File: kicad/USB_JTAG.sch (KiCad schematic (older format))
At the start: 23 parts, among them J1 USB_B, U4 NFM18PS, U5 WE-TVS-824011, U6 FT2232D, U7 6MHz_Crystal, U8 AT93C46DN-SH

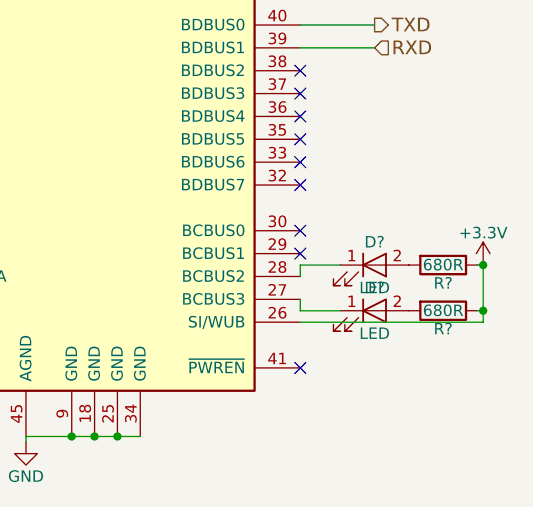
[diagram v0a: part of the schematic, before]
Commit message: Layout changes [In progress]
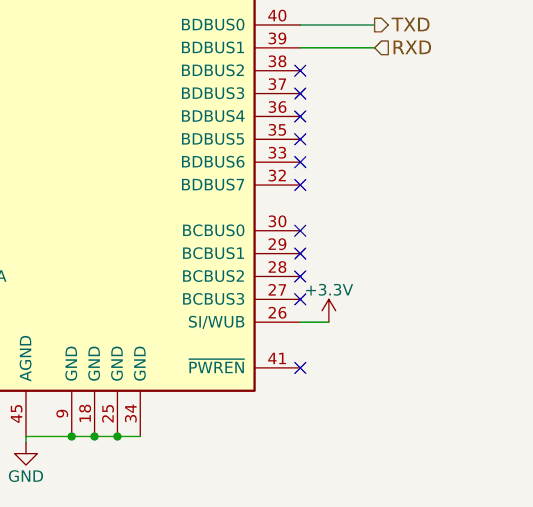
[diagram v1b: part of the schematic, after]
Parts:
- removed D? (x2): LED, Footprints_LJ:Mini_TopLed_SMD, symbol LED
- removed R? (x2): 680R, Resistors_SMD:R_0603_HandSoldering, symbol R
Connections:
- no-connect marks 19 -> 21
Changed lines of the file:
@@
 $EndComp
 $Comp
-L GND #PWR084
+L GND #PWR082
 U 1 1 595D2BC3
 P 1400 3350
-F 0 "#PWR084" H 1400 3100 50  0001 C CNN
+F 0 "#PWR082" H 1400 3100 50  0001 C CNN
 F 1 "GND" H 1400 3200 50  0000 C CNN
 F 2 "" H 1400 3350 50  0001 C CNN
@@
 $EndComp
 $Comp
-L GND #PWR085
+L GND #PWR083
 U 1 1 595D2BF4
 P 5975 5550
-F 0 "#PWR085" H 5975 5300 50  0001 C CNN
+F 0 "#PWR083" H 5975 5300 50  0001 C CNN
 F 1 "GND" H 5975 5400 50  0000 C CNN
 F 2 "" H 5975 5550 50  0001 C CNN
@@
 $EndComp
 $Comp
-L GND #PWR086
+L GND #PWR084
 U 1 1 595D2BFA
 P 5375 5025
-F 0 "#PWR086" H 5375 4775 50  0001 C CNN
+F 0 "#PWR084" H 5375 4775 50  0001 C CNN
 F 1 "GND" H 5375 4875 50  0000 C CNN
 F 2 "" H 5375 5025 50  0001 C CNN
@@
 $EndComp
 $Comp
-L GND #PWR087
+L GND #PWR085
 U 1 1 595D2C07
 P 5075 2425
-F 0 "#PWR087" H 5075 2175 50  0001 C CNN
+F 0 "#PWR085" H 5075 2175 50  0001 C CNN
 F 1 "GND" H 5075 2275 50  0000 C CNN
 F 2 "" H 5075 2425 50  0001 C CNN
@@
 $EndComp
 $Comp
-L GND #PWR088
+L GND #PWR086
 U 1 1 595D2C1A
 P 5450 2025
-F 0 "#PWR088" H 5450 1775 50  0001 C CNN
+F 0 "#PWR086" H 5450 1775 50  0001 C CNN
 F 1 "GND" H 5450 1875 50  0000 C CNN
 F 2 "" H 5450 2025 50  0001 C CNN
@@
 $EndComp
 $Comp
-L +3.3V #PWR089
+L +3.3V #PWR087
 U 1 1 595E0732
 P 6375 1825
-F 0 "#PWR089" H 6375 1675 50  0001 C CNN
+F 0 "#PWR087" H 6375 1675 50  0001 C CNN
 F 1 "+3.3V" H 6375 1965 50  0000 C CNN
 F 2 "" H 6375 1825 50  0001 C CNN
@@
 $EndComp
 $Comp
-L GND #PWR090
+L GND #PWR088
 U 1 1 595E26E9
 P 2800 2450
-F 0 "#PWR090" H 2800 2200 50  0001 C CNN
+F 0 "#PWR088" H 2800 2200 50  0001 C CNN
 F 1 "GND" H 2800 2300 50  0000 C CNN
 F 2 "" H 2800 2450 50  0001 C CNN
@@
 $EndComp
 $Comp
-L GND #PWR091
+L GND #PWR089
 U 1 1 595E2C1D
 P 2075 3400
-F 0 "#PWR091" H 2075 3150 50  0001 C CNN
+F 0 "#PWR089" H 2075 3150 50  0001 C CNN
 F 1 "GND" H 2075 3250 50  0000 C CNN
 F 2 "" H 2075 3400 50  0001 C CNN
@@
 $EndComp
 $Comp
-L GND #PWR092
+L GND #PWR090
 U 1 1 595E6BEC
 P 2200 2250
-F 0 "#PWR092" H 2200 2000 50  0001 C CNN
+F 0 "#PWR090" H 2200 2000 50  0001 C CNN
 F 1 "GND" H 2200 2100 50  0000 C CNN
 F 2 "" H 2200 2250 50  0001 C CNN
@@
 $EndComp
 $Comp
-L GND #PWR093
+L GND #PWR091
 U 1 1 5961A2DE
 P 2400 3400
-F 0 "#PWR093" H 2400 3150 50  0001 C CNN
+F 0 "#PWR091" H 2400 3150 50  0001 C CNN
 F 1 "GND" H 2400 3250 50  0000 C CNN
 F 2 "" H 2400 3400 50  0001 C CNN
@@
 ~RESET
 $Comp
-L +3.3V #PWR094
+L +3.3V #PWR092
 U 1 1 5964E324
 P 3850 4225
-F 0 "#PWR094" H 3850 4075 50  0001 C CNN
+F 0 "#PWR092" H 3850 4075 50  0001 C CNN
 F 1 "+3.3V" H 3850 4365 50  0000 C CNN
 F 2 "" H 3850 4225 50  0001 C CNN
@@
 $EndComp
 $Comp
-L +3.3V #PWR095
+L +3.3V #PWR093
 U 1 1 5964E7A5
 P 2750 4650
-F 0 "#PWR095" H 2750 4500 50  0001 C CNN
+F 0 "#PWR093" H 2750 4500 50  0001 C CNN
 F 1 "+3.3V" H 2750 4790 50  0000 C CNN
 F 2 "" H 2750 4650 50  0001 C CNN
@@
 $EndComp
 $Comp
-L GND #PWR096
+L GND #PWR094
 U 1 1 5964E8AB
 P 2750 4950
-F 0 "#PWR096" H 2750 4700 50  0001 C CNN
+F 0 "#PWR094" H 2750 4700 50  0001 C CNN
 F 1 "GND" H 2750 4800 50  0000 C CNN
 F 2 "" H 2750 4950 50  0001 C CNN
@@
 $EndComp
 $Comp
-L +5V #PWR097
+L +5V #PWR095
 U 1 1 5968BBC0
 P 2075 1925
-F 0 "#PWR097" H 2075 1775 50  0001 C CNN
+F 0 "#PWR095" H 2075 1775 50  0001 C CNN
 F 1 "+5V" H 2075 2065 50  0000 C CNN
 F 2 "" H 2075 1925 50  0001 C CNN
@@
 $EndComp
 $Comp
-L +5V #PWR098
+L +5V #PWR096
 U 1 1 596B00B1
 P 6125 1700
-F 0 "#PWR098" H 6125 1550 50  0001 C CNN
+F 0 "#PWR096" H 6125 1550 50  0001 C CNN
 F 1 "+5V" H 6125 1840 50  0000 C CNN
 F 2 "" H 6125 1700 50  0001 C CNN
@@
 $EndComp
 $Comp
-L +5V #PWR099
+L +5V #PWR097
 U 1 1 596CAD7A
 P 4950 1675
-F 0 "#PWR099" H 4950 1525 50  0001 C CNN
+F 0 "#PWR097" H 4950 1525 50  0001 C CNN
 F 1 "+5V" H 4950 1815 50  0000 C CNN
 F 2 "" H 4950 1675 50  0001 C CNN
@@
 Connection ~ 4550 4325
 $Comp
-L GND #PWR0100
+L GND #PWR098
 U 1 1 5973DDBE
 P 4550 4350
-F 0 "#PWR0100" H 4550 4100 50  0001 C CNN
+F 0 "#PWR098" H 4550 4100 50  0001 C CNN
 F 1 "GND" H 4550 4200 50  0000 C CNN
 F 2 "" H 4550 4350 50  0001 C CNN
@@
 	7175 3525 7350 3525
 $Comp
-L +3.3V #PWR?
+L +3.3V #PWR099
 U 1 1 59BBED1D
 P 7350 3525
-F 0 "#PWR?" H 7350 3375 50  0001 C CNN
+F 0 "#PWR099" H 7350 3375 50  0001 C CNN
 F 1 "+3.3V" H 7350 3665 50  0000 C CNN
 F 2 "" H 7350 3525 50  0001 C CNN
@@
 	1    0    0    -1
 $EndComp
-Wire Wire Line
-	7975 4775 7950 4775
-$Comp
-L R R?
-U 1 1 59BBFFB0
-P 7800 4775
-F 0 "R?" V 7880 4775 50  0000 C CNN
-F 1 "680R" V 7800 4775 50  0000 C CNN
-F 2 "Resistors_SMD:R_0603_HandSoldering" V 7730 4775 50  0001 C CNN
-F 3 "" H 7800 4775 50  0001 C CNN
-	1    7800 4775
-	0    1    1    0
-$EndComp
-$Comp
-L LED D?
-U 1 1 59BBFFB9
-P 7500 4975
-F 0 "D?" H 7500 5075 50  0000 C CNN
-F 1 "LED" H 7500 4875 50  0000 C CNN
-F 2 "Footprints_LJ:Mini_TopLed_SMD" H 7500 4975 50  0001 C CNN
-F 3 "" H 7500 4975 50  0001 C CNN
-	1    7500 4975
-	1    0    0    -1
-$EndComp
-Wire Wire Line
-	7975 4975 7950 4975
-$Comp
-L R R?
-U 1 1 59BBFFC7
-P 7800 4975
-F 0 "R?" V 7880 4975 50  0000 C CNN
-F 1 "680R" V 7800 4975 50  0000 C CNN
-F 2 "Resistors_SMD:R_0603_HandSoldering" V 7730 4975 50  0001 C CNN
-F 3 "" H 7800 4975 50  0001 C CNN
-	1    7800 4975
-	0    1    1    0
-$EndComp
-$Comp
-L LED D?
-U 1 1 59BBFFA2
-P 7500 4775
-F 0 "D?" H 7500 4875 50  0000 C CNN
-F 1 "LED" H 7500 4675 50  0000 C CNN
-F 2 "Footprints_LJ:Mini_TopLed_SMD" H 7500 4775 50  0001 C CNN
-F 3 "" H 7500 4775 50  0001 C CNN
-	1    7500 4775
-	1    0    0    -1
-$EndComp
-Wire Wire Line
-	7175 4775 7175 4825
-Wire Wire Line
-	7175 4925 7175 4975
-$Comp
-L +3.3V #PWR?
-U 1 1 59BC15FC
-P 7975 4775
-F 0 "#PWR?" H 7975 4625 50  0001 C CNN
-F 1 "+3.3V" H 7975 4915 50  0000 C CNN
-F 2 "" H 7975 4775 50  0001 C CNN
-F 3 "" H 7975 4775 50  0001 C CNN
-	1    7975 4775
-	1    0    0    -1
-$EndComp
-Wire Wire Line
-	7175 4975 7350 4975
-Wire Wire Line
-	7175 4775 7350 4775
-Wire Wire Line
-	7975 4775 7975 5025
-Connection ~ 7975 4775
-Wire Wire Line
-	7975 5025 7175 5025
-Connection ~ 7975 4975
+NoConn ~ 7175 4825
+NoConn ~ 7175 4925
+Wire Wire Line
+	7175 5025 7300 5025
+$Comp
+L +3.3V #PWR0100
+U 1 1 59C1476A
+P 7300 5025
+F 0 "#PWR0100" H 7300 4875 50  0001 C CNN
+F 1 "+3.3V" H 7300 5165 50  0000 C CNN
+F 2 "" H 7300 5025 50  0001 C CNN
+F 3 "" H 7300 5025 50  0001 C CNN
+	1    7300 5025
+	1    0    0    -1
+$EndComp
 $EndSCHEMATC

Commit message: Remove design errors and changes some footprints [to review]
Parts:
- U7: footprint Crystals:Crystal_HC49-U_Vertical -> Crystals:Crystal_SMD_HC49-SD
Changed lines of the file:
@@
 $EndComp
 $Comp
-L GND #PWR026
+L GND #PWR027
 U 1 1 595D2BC3
 P 1400 3350
-F 0 "#PWR026" H 1400 3100 50  0001 C CNN
+F 0 "#PWR027" H 1400 3100 50  0001 C CNN
 F 1 "GND" H 1400 3200 50  0000 C CNN
 F 2 "" H 1400 3350 50  0001 C CNN
@@
 F 0 "U7" V 5625 4550 60  0000 C CNN
 F 1 "6MHz_Crystal" V 5550 4350 60  0000 C CNN
-F 2 "Crystals:Crystal_HC49-U_Vertical" H 5400 4200 60  0001 C CNN
+F 2 "Crystals:Crystal_SMD_HC49-SD" H 5400 4200 60  0001 C CNN
 F 3 "" H 5400 4200 60  0001 C CNN
 	1    5400 4200
@@
 $EndComp
 $Comp
-L GND #PWR027
+L GND #PWR028
 U 1 1 595D2BF4
 P 5975 5550
-F 0 "#PWR027" H 5975 5300 50  0001 C CNN
+F 0 "#PWR028" H 5975 5300 50  0001 C CNN
 F 1 "GND" H 5975 5400 50  0000 C CNN
 F 2 "" H 5975 5550 50  0001 C CNN
@@
 $EndComp
 $Comp
-L GND #PWR028
+L GND #PWR029
 U 1 1 595D2BFA
 P 5375 5025
-F 0 "#PWR028" H 5375 4775 50  0001 C CNN
+F 0 "#PWR029" H 5375 4775 50  0001 C CNN
 F 1 "GND" H 5375 4875 50  0000 C CNN
 F 2 "" H 5375 5025 50  0001 C CNN
@@
 $EndComp
 $Comp
-L GND #PWR029
+L GND #PWR030
 U 1 1 595D2C07
 P 5075 2425
-F 0 "#PWR029" H 5075 2175 50  0001 C CNN
+F 0 "#PWR030" H 5075 2175 50  0001 C CNN
 F 1 "GND" H 5075 2275 50  0000 C CNN
 F 2 "" H 5075 2425 50  0001 C CNN
@@
 $EndComp
 $Comp
-L GND #PWR030
+L GND #PWR031
 U 1 1 595D2C1A
 P 5450 2025
-F 0 "#PWR030" H 5450 1775 50  0001 C CNN
+F 0 "#PWR031" H 5450 1775 50  0001 C CNN
 F 1 "GND" H 5450 1875 50  0000 C CNN
 F 2 "" H 5450 2025 50  0001 C CNN
@@
 $EndComp
 $Comp
-L +3.3V #PWR031
+L +3.3V #PWR032
 U 1 1 595E0732
 P 6375 1825
-F 0 "#PWR031" H 6375 1675 50  0001 C CNN
+F 0 "#PWR032" H 6375 1675 50  0001 C CNN
 F 1 "+3.3V" H 6375 1965 50  0000 C CNN
 F 2 "" H 6375 1825 50  0001 C CNN
@@
 $EndComp
 $Comp
-L GND #PWR032
+L GND #PWR033
 U 1 1 595E26E9
 P 2800 2450
-F 0 "#PWR032" H 2800 2200 50  0001 C CNN
+F 0 "#PWR033" H 2800 2200 50  0001 C CNN
 F 1 "GND" H 2800 2300 50  0000 C CNN
 F 2 "" H 2800 2450 50  0001 C CNN
@@
 $EndComp
 $Comp
-L GND #PWR033
+L GND #PWR034
 U 1 1 595E2C1D
 P 2075 3400
-F 0 "#PWR033" H 2075 3150 50  0001 C CNN
+F 0 "#PWR034" H 2075 3150 50  0001 C CNN
 F 1 "GND" H 2075 3250 50  0000 C CNN
 F 2 "" H 2075 3400 50  0001 C CNN
@@
 $EndComp
 $Comp
-L GND #PWR034
+L GND #PWR035
 U 1 1 595E6BEC
 P 2200 2250
-F 0 "#PWR034" H 2200 2000 50  0001 C CNN
+F 0 "#PWR035" H 2200 2000 50  0001 C CNN
 F 1 "GND" H 2200 2100 50  0000 C CNN
 F 2 "" H 2200 2250 50  0001 C CNN
@@
 $EndComp
 $Comp
-L GND #PWR035
+L GND #PWR036
 U 1 1 5961A2DE
 P 2400 3400
-F 0 "#PWR035" H 2400 3150 50  0001 C CNN
+F 0 "#PWR036" H 2400 3150 50  0001 C CNN
 F 1 "GND" H 2400 3250 50  0000 C CNN
 F 2 "" H 2400 3400 50  0001 C CNN
@@
 ~RESET
 $Comp
-L +3.3V #PWR036
+L +3.3V #PWR037
 U 1 1 5964E324
 P 3850 4225
-F 0 "#PWR036" H 3850 4075 50  0001 C CNN
+F 0 "#PWR037" H 3850 4075 50  0001 C CNN
 F 1 "+3.3V" H 3850 4365 50  0000 C CNN
 F 2 "" H 3850 4225 50  0001 C CNN
@@
 $EndComp
 $Comp
-L +3.3V #PWR037
+L +3.3V #PWR038
 U 1 1 5964E7A5
 P 2750 4650
-F 0 "#PWR037" H 2750 4500 50  0001 C CNN
+F 0 "#PWR038" H 2750 4500 50  0001 C CNN
 F 1 "+3.3V" H 2750 4790 50  0000 C CNN
 F 2 "" H 2750 4650 50  0001 C CNN
@@
 $EndComp
 $Comp
-L GND #PWR038
+L GND #PWR039
 U 1 1 5964E8AB
 P 2750 4950
-F 0 "#PWR038" H 2750 4700 50  0001 C CNN
+F 0 "#PWR039" H 2750 4700 50  0001 C CNN
 F 1 "GND" H 2750 4800 50  0000 C CNN
 F 2 "" H 2750 4950 50  0001 C CNN
@@
 $EndComp
 $Comp
-L +5V #PWR039
+L +5V #PWR040
 U 1 1 5968BBC0
 P 2075 1925
-F 0 "#PWR039" H 2075 1775 50  0001 C CNN
+F 0 "#PWR040" H 2075 1775 50  0001 C CNN
 F 1 "+5V" H 2075 2065 50  0000 C CNN
 F 2 "" H 2075 1925 50  0001 C CNN
@@
 $EndComp
 $Comp
-L +5V #PWR040
+L +5V #PWR041
 U 1 1 596B00B1
 P 6125 1700
-F 0 "#PWR040" H 6125 1550 50  0001 C CNN
+F 0 "#PWR041" H 6125 1550 50  0001 C CNN
 F 1 "+5V" H 6125 1840 50  0000 C CNN
 F 2 "" H 6125 1700 50  0001 C CNN
@@
 $EndComp
 $Comp
-L +5V #PWR041
+L +5V #PWR042
 U 1 1 596CAD7A
 P 4950 1675
-F 0 "#PWR041" H 4950 1525 50  0001 C CNN
+F 0 "#PWR042" H 4950 1525 50  0001 C CNN
 F 1 "+5V" H 4950 1815 50  0000 C CNN
 F 2 "" H 4950 1675 50  0001 C CNN
@@
 Connection ~ 4550 4325
 $Comp
-L GND #PWR042
+L GND #PWR043
 U 1 1 5973DDBE
 P 4550 4350
-F 0 "#PWR042" H 4550 4100 50  0001 C CNN
+F 0 "#PWR043" H 4550 4100 50  0001 C CNN
 F 1 "GND" H 4550 4200 50  0000 C CNN
 F 2 "" H 4550 4350 50  0001 C CNN
@@
 	7175 3525 7350 3525
 $Comp
-L +3.3V #PWR043
+L +3.3V #PWR044
 U 1 1 59BBED1D
 P 7350 3525
-F 0 "#PWR043" H 7350 3375 50  0001 C CNN
+F 0 "#PWR044" H 7350 3375 50  0001 C CNN
 F 1 "+3.3V" H 7350 3665 50  0000 C CNN
 F 2 "" H 7350 3525 50  0001 C CNN
@@
 	7175 5025 7300 5025
 $Comp
-L +3.3V #PWR044
+L +3.3V #PWR045
 U 1 1 59C1476A
 P 7300 5025
-F 0 "#PWR044" H 7300 4875 50  0001 C CNN
+F 0 "#PWR045" H 7300 4875 50  0001 C CNN
 F 1 "+3.3V" H 7300 5165 50  0000 C CNN
 F 2 "" H 7300 5025 50  0001 C CNN
